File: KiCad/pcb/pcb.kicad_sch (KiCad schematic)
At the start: 20 parts, among them J1 Jack-DC, J2 Screw_Terminal_01x02, J3 Screw_Terminal_01x02, J4 Screw_Terminal_01x02, J5 Screw_Terminal_01x03, U2 Tauno_Oled_096_SSD1306, U6 PC817

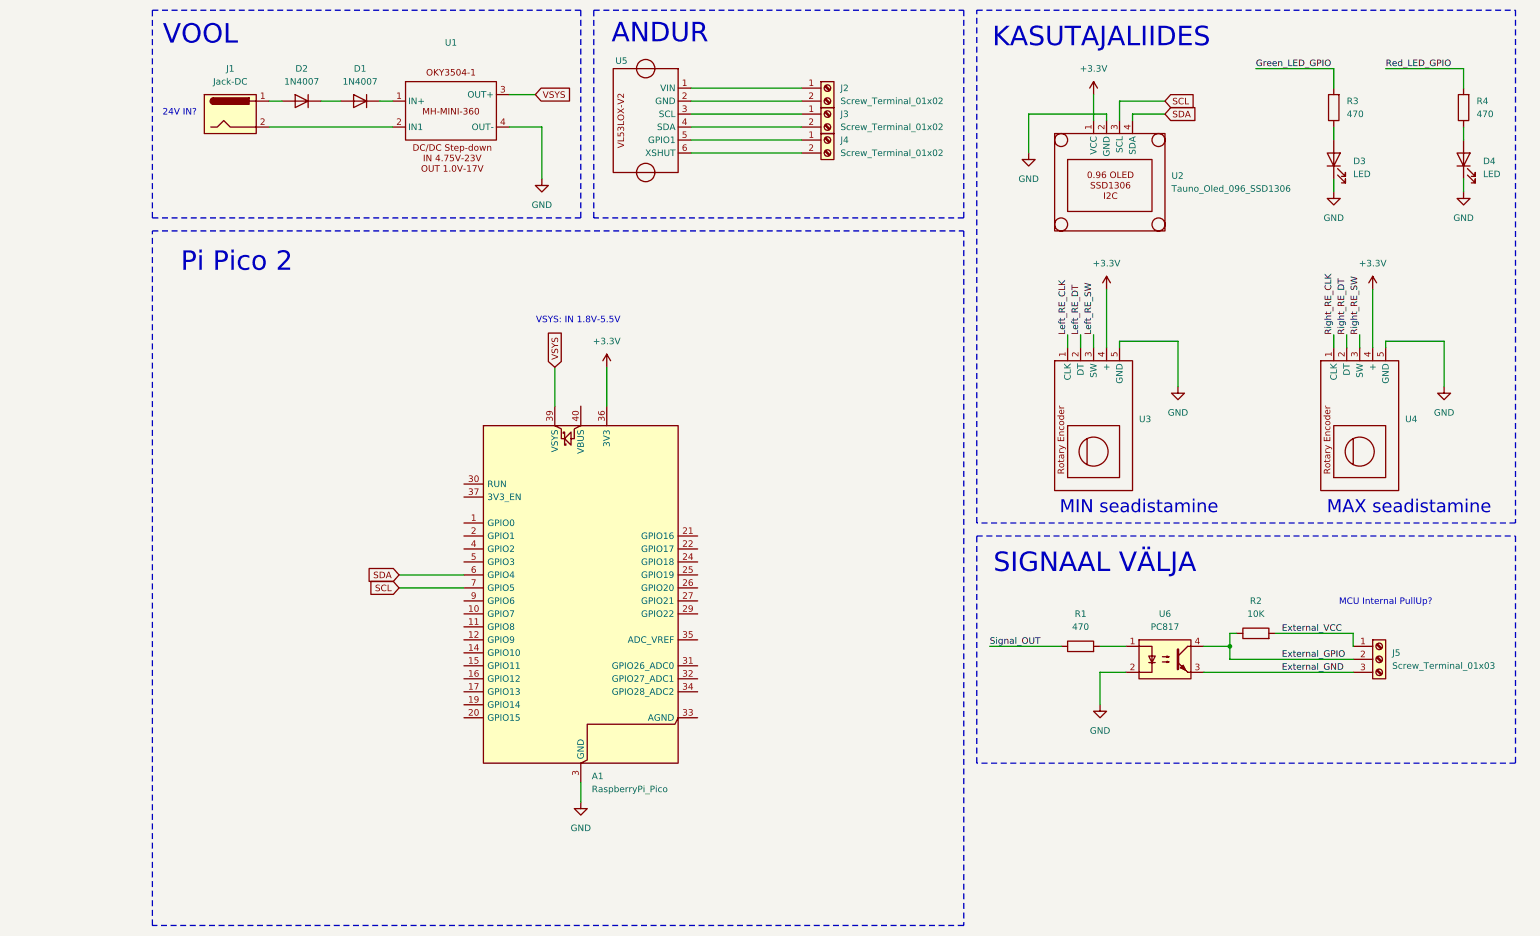
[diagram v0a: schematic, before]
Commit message: kicad files
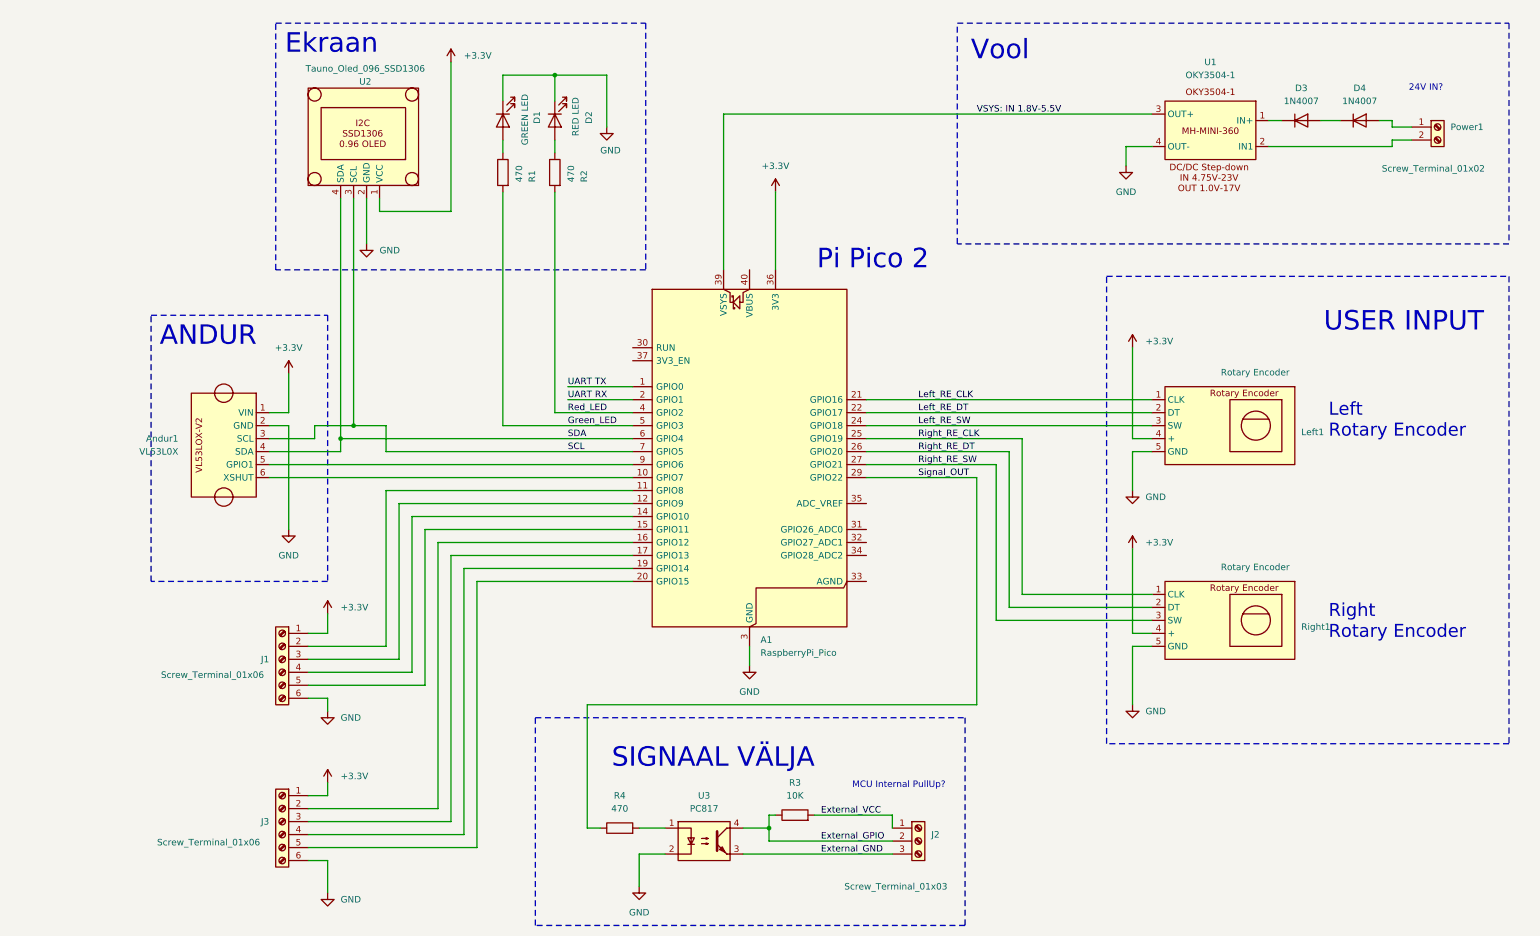
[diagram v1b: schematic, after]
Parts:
- removed J1: Jack-DC, symbol Connector:Jack-DC
- removed J2, J3, J4: Screw_Terminal_01x02, TerminalBlock:TerminalBlock_MaiXu_MX126-5.0-02P_1x02_P5.00mm, symbol Connector:Screw_Terminal_01x02
- removed U3, U4: ~, symbol Tauno_Library:Tauno_Rotary_Encoder
- removed U5: ~, symbol Tauno_Library:Tauno_TOF_VL53LOX
- added Andur1: VL53L0X, TerminalBlock:TerminalBlock_MaiXu_MX126-5.0-06P_1x06_P5.00mm, symbol Tauno_Library:Tauno_TOF_VL53LOX
- added J1, J3: Screw_Terminal_01x06, TerminalBlock:TerminalBlock_MaiXu_MX126-5.0-06P_1x06_P5.00mm, symbol Connector:Screw_Terminal_01x06
- added Left1, Right1: Rotary Encoder, Taunoe_footprints:Tauno_Rotary_Encoder, symbol Tauno_Library:Tauno_Rotary_Encoder
- added Power1: Screw_Terminal_01x02, TerminalBlock_MetzConnect:TerminalBlock_MetzConnect_Type011_RT05502HBLC_1x02_P5.00mm_Horizontal, symbol Connector:Screw_Terminal_01x02
- A1: footprint Module:RaspberryPi_Pico_Common_SMD -> Module:RaspberryPi_Pico_Common_Unspecified
- D1: renamed from D3; value LED -> GREEN LED; footprint (none) -> LED_THT:LED_Rectangular_W5.0mm_H2.0mm
- D2: renamed from D4; value LED -> RED LED; footprint (none) -> LED_THT:LED_Rectangular_W5.0mm_H2.0mm
- J2: renamed from J5; footprint (none) -> TerminalBlock:TerminalBlock_MaiXu_MX126-5.0-03P_1x03_P5.00mm
- R1: renamed from R3; footprint (none) -> Resistor_THT:R_Axial_DIN0207_L6.3mm_D2.5mm_P10.16mm_Horizontal
- R2: renamed from R4; footprint (none) -> Resistor_THT:R_Axial_DIN0207_L6.3mm_D2.5mm_P10.16mm_Horizontal
- R3: renamed from R2; footprint (none) -> Resistor_THT:R_Axial_DIN0207_L6.3mm_D2.5mm_P10.16mm_Horizontal
- R4: renamed from R1; footprint (none) -> Resistor_THT:R_Axial_DIN0207_L6.3mm_D2.5mm_P10.16mm_Horizontal
- U1: value ~ -> OKY3504-1; footprint (none) -> Taunoe_footprints:Tauno_OKY3504
- renumbered D1 to D3, D2 to D4, U6 to U3
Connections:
- net Green_LED_GPIO is gone; now on net Green_LED: R1.2
- net Red_LED_GPIO is gone; now on net Red_LED: R2.2
- net +3.3V: now also Andur1.1 (VIN), J1.1 (Pin_1), J3.1 (Pin_1), Left1.4 (+), Right1.4 (+)
- net GND: now also Andur1.2 (GND), J1.6 (Pin_6), J3.6 (Pin_6), Left1.5 (GND), Right1.5 (GND)
- net Left_RE_CLK: now also A1.21 (GPIO16), Left1.1 (CLK)
- net Left_RE_DT: now also A1.22 (GPIO17), Left1.2 (DT)
- net Left_RE_SW: now also A1.24 (GPIO18), Left1.3 (SW)
- net Right_RE_CLK: now also A1.25 (GPIO19), Right1.1 (CLK)
- net Right_RE_DT: now also A1.26 (GPIO20), Right1.2 (DT)
- net Right_RE_SW: now also A1.27 (GPIO21), Right1.3 (SW)
- net SCL: now also Andur1.3 (SCL)
- net SDA: now also Andur1.4 (SDA)
- net Signal_OUT: now also A1.29 (GPIO22)
- net at D4.2 (A): now also Power1.1 (Pin_1)
- net at U1.2 (IN1): now also Power1.2 (Pin_2)
- net UART TX: now reaches A1.1 (GPIO0)
- net at A1.10 (GPIO7): now also Andur1.6 (XSHUT)
- net at A1.11 (GPIO8): now also J1.2 (Pin_2)
- net at A1.12 (GPIO9): now also J1.3 (Pin_3)
- net at A1.14 (GPIO10): now also J1.4 (Pin_4)
- net at A1.15 (GPIO11): now also J1.5 (Pin_5)
- net at A1.16 (GPIO12): now also J3.2 (Pin_2)
- net at A1.17 (GPIO13): now also J3.3 (Pin_3)
- net at A1.19 (GPIO14): now also J3.4 (Pin_4)
- net UART RX: now reaches A1.2 (GPIO1)
- net at A1.20 (GPIO15): now also J3.5 (Pin_5)
- net Red_LED: now reaches A1.4 (GPIO2)
- net Green_LED: now reaches A1.5 (GPIO3)
- net at A1.9 (GPIO6): now also Andur1.5 (GPIO1)
- net VSYS renamed VSYS: IN 1.8V-5.5V
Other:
- note added: "Ekraan"
- note added: "Left Rotary Encoder"
- note added: "Right Rotary Encoder"
- note added: "USER INPUT"
- note added: "Vool"
- note removed: "KASUTAJALIIDES"
- note removed: "MAX seadistamine"
- note removed: "MIN seadistamine"
- note removed: "VOOL"
- note removed: "VSYS: IN 1.8V-5.5V"
- title: Pi Pico Andur -> Anduri PCB skeem
- moved on the sheet: A1, D1, D2, D3, D4, J2, R1, R2, R3, R4, U3

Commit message: kicad files
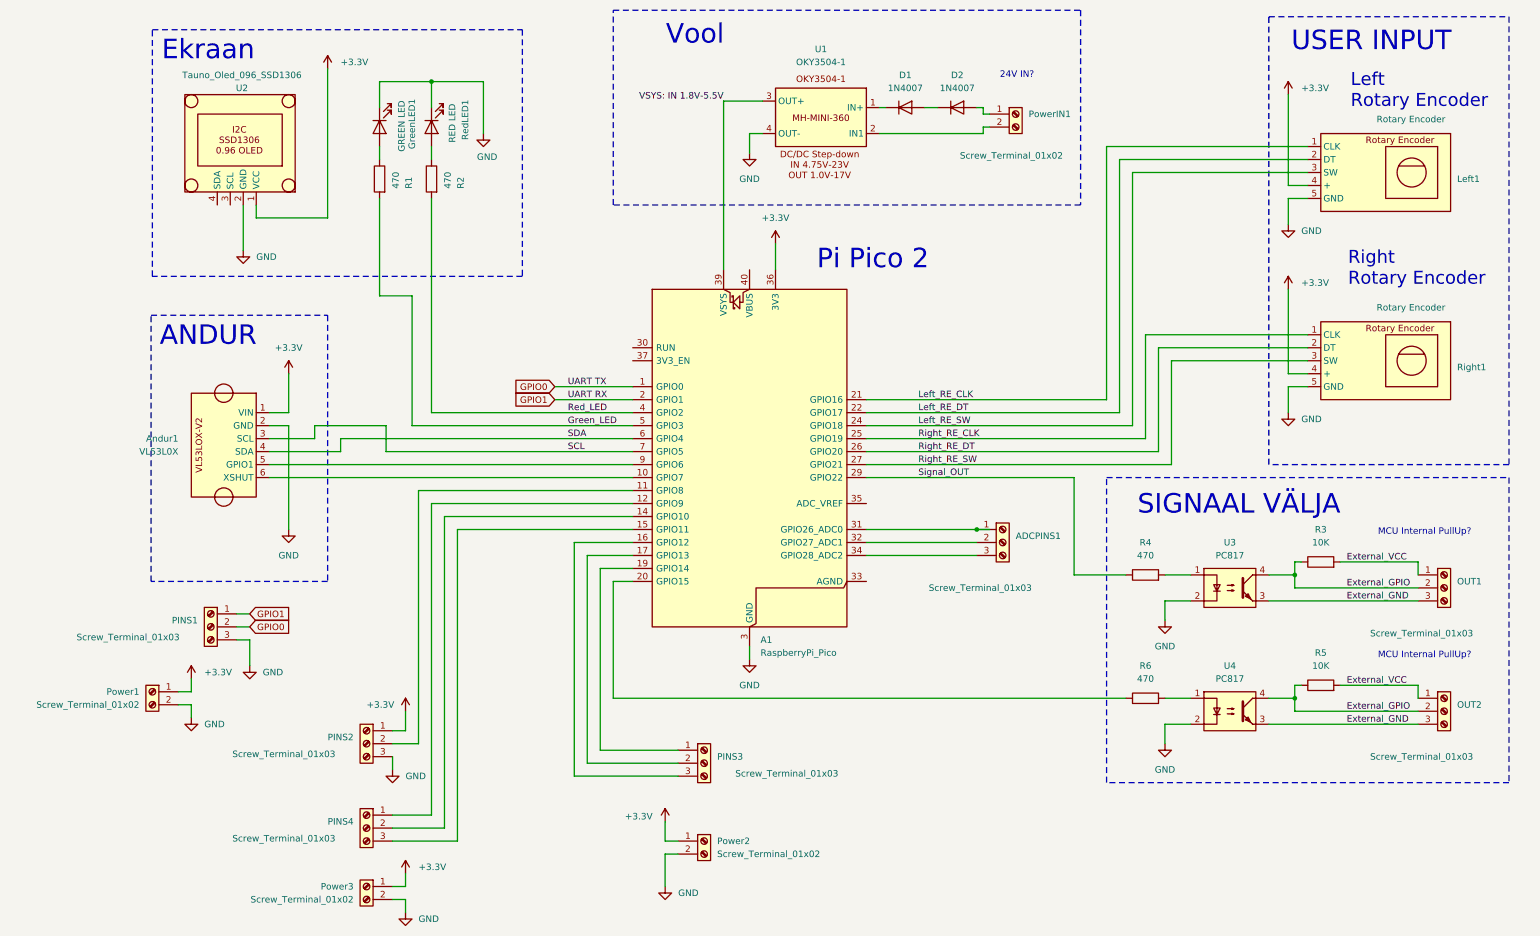
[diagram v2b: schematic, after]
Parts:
- removed J1, J3: Screw_Terminal_01x06, TerminalBlock:TerminalBlock_MaiXu_MX126-5.0-06P_1x06_P5.00mm, symbol Connector:Screw_Terminal_01x06
- added ADCPINS1, OUT2, PINS1, PINS2, PINS3, PINS4: Screw_Terminal_01x03, TerminalBlock:TerminalBlock_MaiXu_MX126-5.0-03P_1x03_P5.00mm, symbol Connector:Screw_Terminal_01x03
- added Power1, Power2, Power3: Screw_Terminal_01x02, TerminalBlock:TerminalBlock_MaiXu_MX126-5.0-02P_1x02_P5.00mm, symbol Connector:Screw_Terminal_01x02
- added R5: 10K, Resistor_THT:R_Axial_DIN0207_L6.3mm_D2.5mm_P10.16mm_Horizontal, symbol Device:R
- added R6: 470, Resistor_THT:R_Axial_DIN0207_L6.3mm_D2.5mm_P10.16mm_Horizontal, symbol Device:R
- added U4: PC817, Package_DIP:DIP-4_W7.62mm, symbol Isolator:PC817
- A1: footprint Module:RaspberryPi_Pico_Common_Unspecified -> Module:RaspberryPi_Pico_W_SMD_HandSolder
- PowerIN1: renamed from Power1; footprint TerminalBlock_MetzConnect:TerminalBlock_MetzConnect_Type011_RT05502HBLC_1x02_P5.00mm_Horizontal -> TerminalBlock:TerminalBlock_MaiXu_MX126-5.0-02P_1x02_P5.00mm
- renumbered D3 to D1, D4 to D2, D1 to GreenLED1, J2 to OUT1, D2 to RedLED1
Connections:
- net +3.3V: now also PINS2.1 (Pin_1), Power1.1 (Pin_1), Power2.1 (Pin_1), Power3.1 (Pin_1)
- net External_GND: now also OUT2.3 (Pin_3), U4.3
- net External_GPIO: now also OUT2.2 (Pin_2), R5.1, U4.4
- net External_VCC: now also OUT2.1 (Pin_1), R5.2
- net GND: now also PINS1.3 (Pin_3), PINS2.3 (Pin_3), Power1.2 (Pin_2), Power2.2 (Pin_2), Power3.2 (Pin_2), U4.2
- net SCL: no longer U2.3 (SCL)
- net SDA: no longer U2.4 (SDA)
- net at A1.11 (GPIO8): now also PINS2.2 (Pin_2)
- net at A1.12 (GPIO9): now also PINS4.1 (Pin_1)
- net at A1.14 (GPIO10): now also PINS4.2 (Pin_2)
- net at A1.15 (GPIO11): now also PINS4.3 (Pin_3)
- net at A1.16 (GPIO12): now also PINS3.3 (Pin_3)
- net at A1.17 (GPIO13): now also PINS3.2 (Pin_2)
- net at A1.19 (GPIO14): now also PINS3.1 (Pin_1)
- net at A1.20 (GPIO15): now also R6.1
- net at A1.31 (GPIO26_ADC0): now also ADCPINS1.1 (Pin_1)
- net at A1.32 (GPIO27_ADC1): now also ADCPINS1.2 (Pin_2)
- net at A1.34 (GPIO28_ADC2): now also ADCPINS1.3 (Pin_3)
- net UART RX renamed GPIO1
- net GPIO1: now also PINS1.1 (Pin_1)
- net UART TX renamed GPIO0
- net GPIO0: now also PINS1.2 (Pin_2)
- new net: R6.2, U4.1
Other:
- moved on the sheet: D1, D2, GreenLED1, Left1, OUT1, PowerIN1, R1, R2, R3, R4, RedLED1, Right1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
